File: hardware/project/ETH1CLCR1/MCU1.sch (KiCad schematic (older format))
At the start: 42 parts, among them J301 Conn_02x01, J302 20021111-00010T4LF, U301 STM32F765ZGT6, U302 24LC08B-E/MS, U303 HDC1080, Y301 NX3225GD-8MHZ-STD-CRA-3

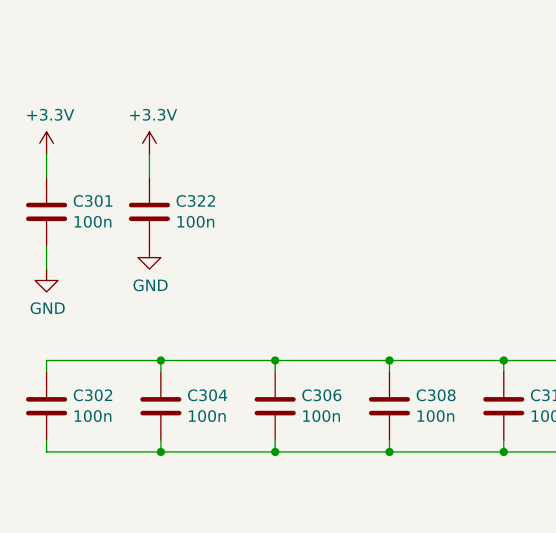
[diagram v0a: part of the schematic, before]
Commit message: PCB layout
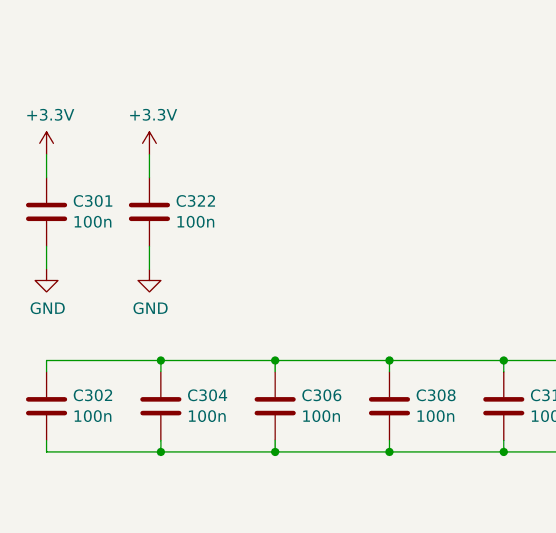
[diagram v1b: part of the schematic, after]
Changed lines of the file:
@@
 L power:GND #PWR0103
 U 1 1 5EFC3E57
-P 1100 10000
-F 0 "#PWR0103" H 1100 9750 50  0001 C CNN
-F 1 "GND" H 1105 9827 50  0000 C CNN
-F 2 "" H 1100 10000 50  0001 C CNN
-F 3 "" H 1100 10000 50  0001 C CNN
-	1    1100 10000
+P 1100 10100
+F 0 "#PWR0103" H 1100 9850 50  0001 C CNN
+F 1 "GND" H 1105 9927 50  0000 C CNN
+F 2 "" H 1100 10100 50  0001 C CNN
+F 3 "" H 1100 10100 50  0001 C CNN
+	1    1100 10100
 	1    0    0    -1
 $EndComp
@@
 Text Label 2700 1500 0    50   ~ 0
 SENS_SDA
+Wire Wire Line
+	1100 10100 1100 10000
 $EndSCHEMATC
